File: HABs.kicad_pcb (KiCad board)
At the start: 2 copper layers, 3 parts, among them IC1 CAM-M8C-0-10, U2 Ai-Thinker-Ra-02

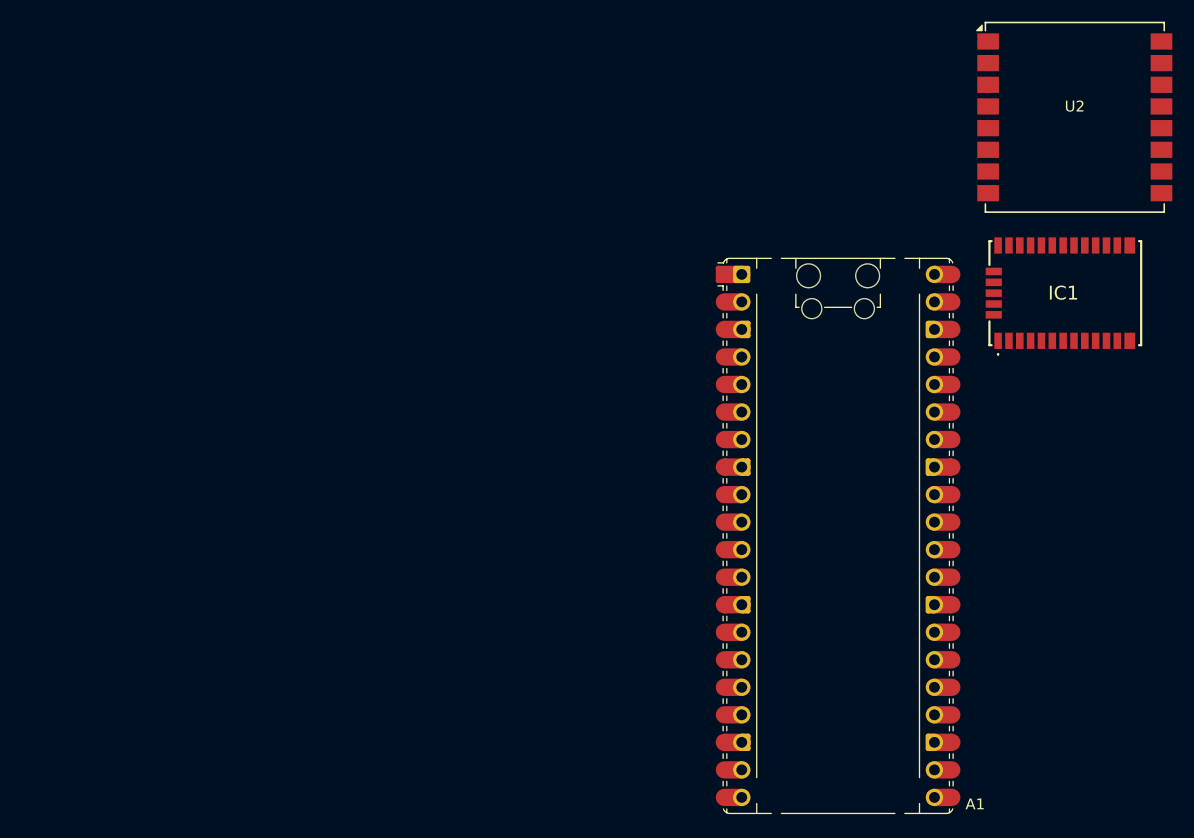
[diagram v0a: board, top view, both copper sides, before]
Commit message: feat: initial PCB layout
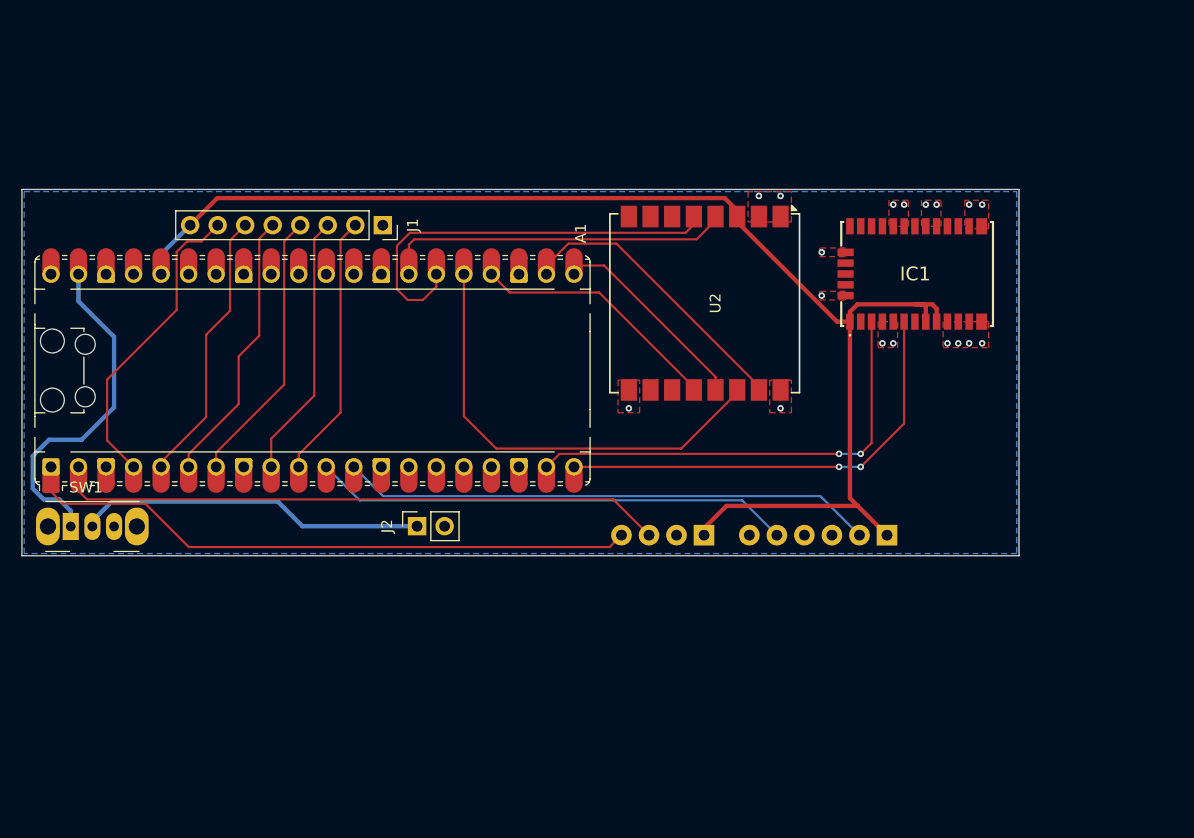
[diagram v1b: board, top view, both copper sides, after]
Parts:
- added J1: Conn_01x08_Pin, Connector_PinSocket_2.54mm:PinSocket_1x08_P2.54mm_Vertical, F.Cu at (72.3, 52.7)
- added J2: Conn_01x02_Pin, Connector_PinSocket_2.54mm:PinSocket_1x02_P2.54mm_Vertical, F.Cu at (75.5, 80.5)
- added SW1: SW_SPDT, Button_Switch_THT:SW_Slide_SPDT_Angled_CK_OS102011MA1Q, F.Cu at (43.5, 80.5)
- added U1: MicroSD, Components:MicroSD, B.Cu at (118.8, 81.3)
- added U3: BMP180, Components:BMP180, B.Cu at (98.1, 76.1)
- moved A1 50.8 mm to (65.8, 66.1), turned to 90 degrees
- moved U2 38.2 mm to (102.0, 59.9), turned to -90 degrees
- moved IC1 13.8 mm to (121.6, 57.2)
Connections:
- net 3.3V renamed +3.3V
- net GPS_ANT renamed /GPS_ANT
- net LORA_SCK renamed /LORA_SCK
- net RX renamed /GPS_RX
- net TX renamed /GPS_TX
- A1 pad 1: unconnected-(A1-GPIO0-Pad1) -> /BMP_SDA
- A1 pad 10: unconnected-(A1-GPIO7-Pad10) -> /SCL
- A1 pad 11: unconnected-(A1-GPIO8-Pad11) -> /SD_MISO
- A1 pad 12: unconnected-(A1-GPIO9-Pad12) -> /SD_CS
- A1 pad 14: SDA -> /SD_CLK
- A1 pad 15: SCL -> /SD_MOSI
- A1 pad 19: unconnected-(A1-GPIO14-Pad19) -> /GPS_SDA
- A1 pad 2: unconnected-(A1-GPIO1-Pad2) -> /BMP_SCL
- A1 pad 20: unconnected-(A1-GPIO15-Pad20) -> /GPS_SCL
- A1 pad 21: LORA_BUSY -> /LORA_MISO
- A1 pad 22: LORA_RESET -> /LORA_CS
- A1 pad 25: LORA_MISO -> /LORA_MOSI
- A1 pad 26: LORA_MOSI -> /LORA_BUSY
- A1 pad 27: LORA_CS -> /LORA_RESET
- A1 pad 4: unconnected-(A1-GPIO2-Pad4) -> /SCK
- A1 pad 5: unconnected-(A1-GPIO3-Pad5) -> /MOSI
- A1 pad 6: unconnected-(A1-GPIO4-Pad6) -> /MISO
- A1 pad 7: unconnected-(A1-GPIO5-Pad7) -> /CS
- A1 pad 9: unconnected-(A1-GPIO6-Pad9) -> /SDA
- IC1 pad 3: SDA -> /GPS_SDA
- IC1 pad 6: SCL -> /GPS_SCL
- U2 pad 13: LORA_MISO -> /LORA_MISO
- U2 pad 14: LORA_MOSI -> /LORA_MOSI
- U2 pad 15: LORA_CS -> /LORA_CS
- U2 pad 4: LORA_RESET -> /LORA_RESET
- U2 pad 5: LORA_BUSY -> /LORA_BUSY
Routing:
- net +3.3V: track 0.00 -> 122.7 mm
- net /BMP_SDA: track 0.00 -> 56.7 mm
- net /BMP_SCL: track 0.00 -> 55.7 mm
- net /SD_CS: track 0.00 -> 49.3 mm
- net /SD_MISO: track 0.00 -> 44.2 mm
- net /GPS_SDA: track 0.00 -> 42.1 mm, vias 0 -> 2
- net /LORA_MOSI: track 0.00 -> 41.9 mm
- net /GPS_SCL: track 0.00 -> 41.5 mm, vias 0 -> 2
- net /LORA_BUSY: track 0.00 -> 39.5 mm
- net Net-(J2-Pin_1): track 0.00 -> 32.1 mm
- net VCC: track 0.00 -> 31.8 mm
- net /LORA_RESET: track 0.00 -> 31.5 mm
- net /SCK: track 0.00 -> 28.3 mm
- net /MOSI: track 0.00 -> 26.3 mm
- net /MISO: track 0.00 -> 26.3 mm
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- added copper zone on B.Cu, net GND
- added copper zone on F.Cu, net GND
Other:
- board outline added: 92 x 33.8 mm
